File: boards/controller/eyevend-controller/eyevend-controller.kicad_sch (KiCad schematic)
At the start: 8 parts, among them J2 Conn_01x03, J3 Conn_01x03, J4 Micro_SD_Card, U1 Pico, U2 _DAC8411

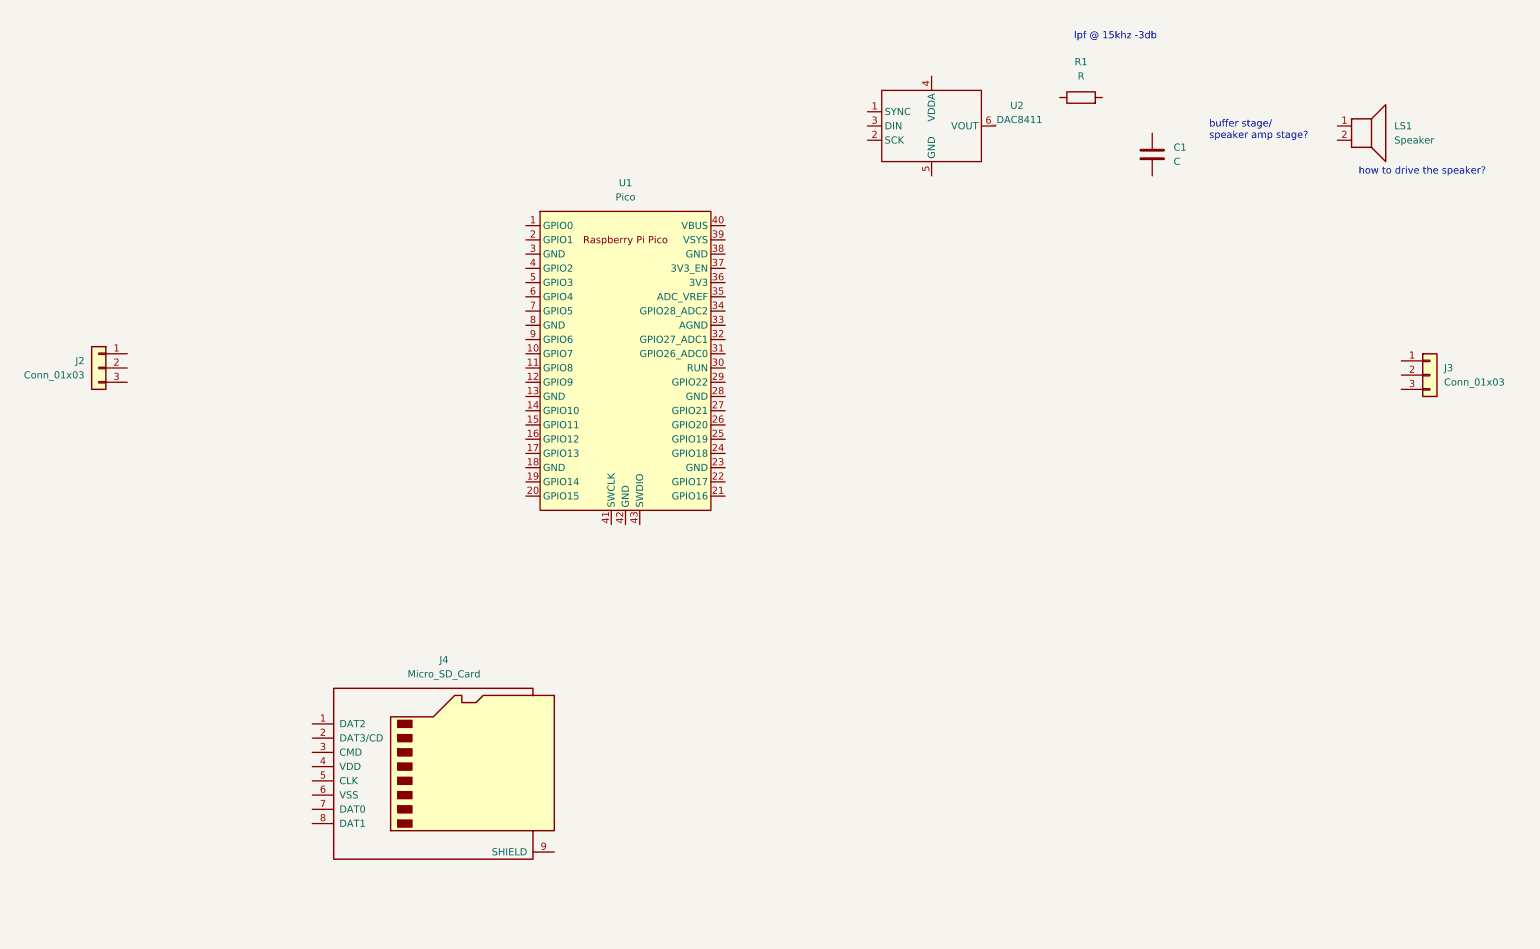
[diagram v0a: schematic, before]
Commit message: updated board
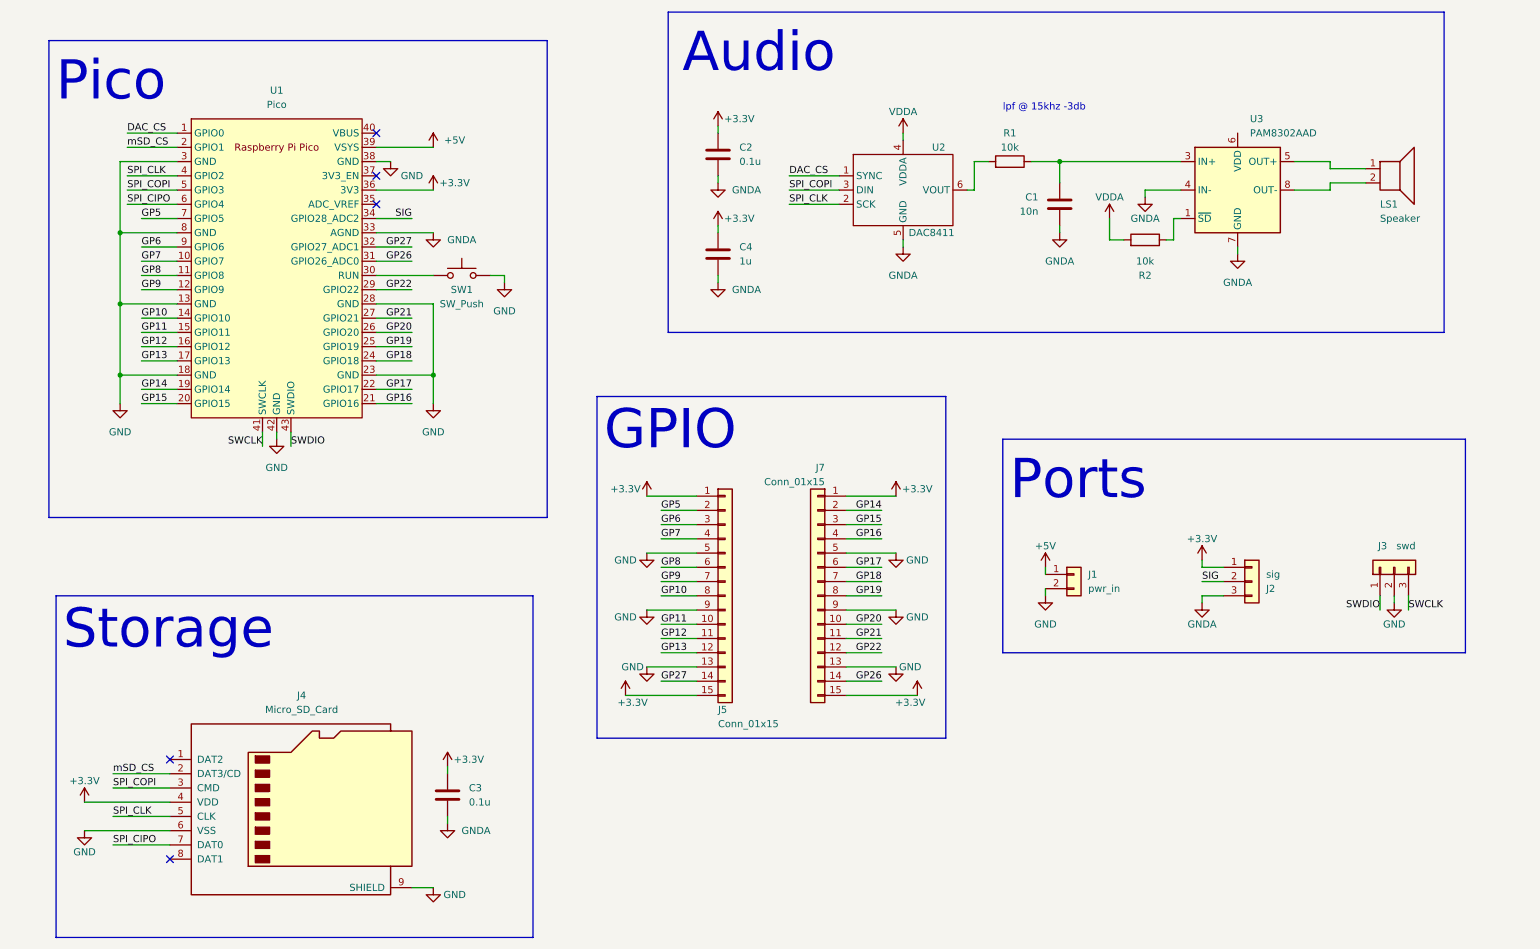
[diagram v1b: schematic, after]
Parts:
- removed U2: _DAC8411, symbol JFHDAC:_DAC8411
- added C2, C3: 0.1u, Capacitor_SMD:C_0402_1005Metric, symbol Device:C
- added C4: 1u, Capacitor_SMD:C_0402_1005Metric, symbol Device:C
- added J1: pwr_in, symbol Connector_Generic:Conn_01x02
- added J5, J7: Conn_01x15, Connector_PinHeader_2.54mm:PinHeader_1x15_P2.54mm_Vertical, symbol Connector_Generic:Conn_01x15
- added R2: 10k, Resistor_SMD:R_0402_1005Metric, symbol Device:R
- added SW1: SW_Push, symbol Switch:SW_Push
- added U2: DAC8411, Package_TO_SOT_SMD:Texas_R-PDSO-G6, symbol JFHDAC:DAC8411
- added U3: PAM8302AAD, symbol Amplifier_Audio:PAM8302AAD
- C1: value C -> 10n; footprint (none) -> Capacitor_SMD:C_0402_1005Metric
- J2: value Conn_01x03 -> sig
- J3: value Conn_01x03 -> swd
- R1: value R -> 10k; footprint (none) -> Resistor_SMD:R_0402_1005Metric
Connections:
- net mSD_CS: now reaches J4.2 (DAT3/CD)
- net mSD_CS: now also U1.2 (GPIO1)
- net SPI_COPI: now reaches J4.3 (CMD)
- net SPI_COPI: now also U1.5 (GPIO3), U2.3 (DIN)
- net +3.3V: now reaches J4.4 (VDD)
- net +3.3V: now also J2.1 (Pin_1), U1.36 (3V3), C2.1, C3.1, C4.1, J5.1 (Pin_1), J5.15 (Pin_15), J7.1 (Pin_1), J7.15 (Pin_15)
- net SPI_CLK: now reaches J4.5 (CLK)
- net SPI_CLK: now also U1.4 (GPIO2), U2.2 (SCK)
- net GND: now reaches J4.6 (VSS)
- net GND: now also J3.2 (Pin_2), J4.9 (SHIELD), U1.13 (GND), U1.18 (GND), U1.23 (GND), U1.28 (GND), U1.3 (GND), U1.38 (GND), U1.42 (GND), U1.8 (GND), J1.2 (Pin_2), J5.13 (Pin_13), J5.5 (Pin_5), J5.9 (Pin_9), J7.13 (Pin_13), J7.5 (Pin_5), J7.9 (Pin_9), SW1.2
- net SPI_CIPO: now reaches J4.7 (DAT0)
- net SPI_CIPO: now also U1.6 (GPIO4)
- net SWDIO: now reaches J3.1 (Pin_1)
- net SWDIO: now also U1.43 (SWDIO)
- net SWCLK: now reaches J3.3 (Pin_3)
- net SWCLK: now also U1.41 (SWCLK)
- net at LS1.1: now also U3.5 (OUT+)
- net at LS1.2: now also U3.8 (OUT-)
- net at R1.1: now also C1.1, U3.3 (IN+)
- net at R1.2: now also U2.6 (VOUT)
- net DAC_CS: now reaches U1.1 (GPIO0)
- net DAC_CS: now also U2.1 (SYNC)
- net GP7: now reaches U1.10 (GPIO7)
- net GP7: now also J5.4 (Pin_4)
- net GP8: now reaches U1.11 (GPIO8)
- net GP8: now also J5.6 (Pin_6)
- net GP9: now reaches U1.12 (GPIO9)
- net GP9: now also J5.7 (Pin_7)
- net GP10: now reaches U1.14 (GPIO10)
- net GP10: now also J5.8 (Pin_8)
- net GP11: now reaches U1.15 (GPIO11)
- net GP11: now also J5.10 (Pin_10)
- net GP12: now reaches U1.16 (GPIO12)
- net GP12: now also J5.11 (Pin_11)
- net GP13: now reaches U1.17 (GPIO13)
- net GP13: now also J5.12 (Pin_12)
- net GP14: now reaches U1.19 (GPIO14)
- net GP14: now also J7.2 (Pin_2)
- net GP15: now reaches U1.20 (GPIO15)
- net GP15: now also J7.3 (Pin_3)
- net GP16: now reaches U1.21 (GPIO16)
- net GP16: now also J7.4 (Pin_4)
- net GP17: now reaches U1.22 (GPIO17)
- net GP17: now also J7.6 (Pin_6)
- net GP18: now reaches U1.24 (GPIO18)
- net GP18: now also J7.7 (Pin_7)
- net GP19: now reaches U1.25 (GPIO19)
- net GP19: now also J7.8 (Pin_8)
- net GP20: now reaches U1.26 (GPIO20)
- net GP20: now also J7.10 (Pin_10)
- net GP21: now reaches U1.27 (GPIO21)
- net GP21: now also J7.11 (Pin_11)
- net GP22: now reaches U1.29 (GPIO22)
- net GP22: now also J7.12 (Pin_12)
- net at U1.30 (RUN): now also SW1.1
- net GP26: now reaches U1.31 (GPIO26_ADC0)
- net GP26: now also J7.14 (Pin_14)
- net GP27: now reaches U1.32 (GPIO27_ADC1)
- net GP27: now also J5.14 (Pin_14)
- net GNDA: now reaches U1.33 (AGND)
- net GNDA: now also C1.2, J2.3 (Pin_3), C2.2, C3.2, C4.2, U2.5 (GND), U3.4 (IN-), U3.7 (GND)
- net SIG: now reaches U1.34 (GPIO28_ADC2)
- net SIG: now also J2.2 (Pin_2)
- net +5V: now reaches U1.39 (VSYS)
- net +5V: now also J1.1 (Pin_1)
- net GP5: now reaches U1.7 (GPIO5)
- net GP5: now also J5.2 (Pin_2)
- net GP6: now reaches U1.9 (GPIO6)
- net GP6: now also J5.3 (Pin_3)
- new net: R2.1, U3.1 (~{SD})
- new net VDDA: R2.2, U2.4 (VDDA)
- no-connect marks 0 -> 5
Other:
- note added: "Audio"
- note added: "GPIO"
- note added: "Pico"
- note added: "Ports"
- note added: "Storage"
- note removed: "buffer stage/ speaker amp stage?"
- note removed: "how to drive the speaker?"
- company: (none) -> JHorwitzDesign
- title: (none) -> EyeVend Controller Board
- moved on the sheet: C1, J4, LS1, R1, U1
